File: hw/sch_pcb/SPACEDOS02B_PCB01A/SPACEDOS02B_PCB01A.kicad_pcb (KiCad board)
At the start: 2 copper layers, 38 x 200 mm, 123 parts, among them J1 MCC-SD, J10 HEADER_1x01, J11 HEADER_1x01, J12 HEADER_1x01, J13 HEADER_1x01, J14 HEADER_1x01, J15 HEADER_1x01, J16 HEADER_1x01, J17 HEADER_1x01, J18 HEADER_1x01, J19 HEADER_2x01_PARALLEL, J2 HEADER_2x01_PARALLEL, J20 HEADER_1x01, J21 HEADER_1x01, J22 HEADER_2x03, J23 HEADER_1x01, J24 HEADER_1x01, J25 HEADER_1x01, J26 HEADER_1x01, J27 HEADER_1x01, J28 SD_Card-FPS009-4200-0, J3 HEADER_2x01_PARALLEL, J4 HEADER_1x01, J5 HEADER_1x01, J6 HEADER_1x01, J7 HEADER_1x01, J8 HEADER_1x01, J9 HEADER_1x01, M6 BMI-S-210-F, M8 BMI-S-210-F, U1 OPA2314, U10 ATMEGA1284P-AU, U11 PCF85263A, U2 OPA2314, U3 ISL21080DIH312Z-TK 1V25, U4 TS7211, U5 TS5A4594, U6 AT24CS64-SSHM, U8 TPS613222ADBV, Y1 1,8432MHz, Y2 ABS07-120-32.768KHZ-T

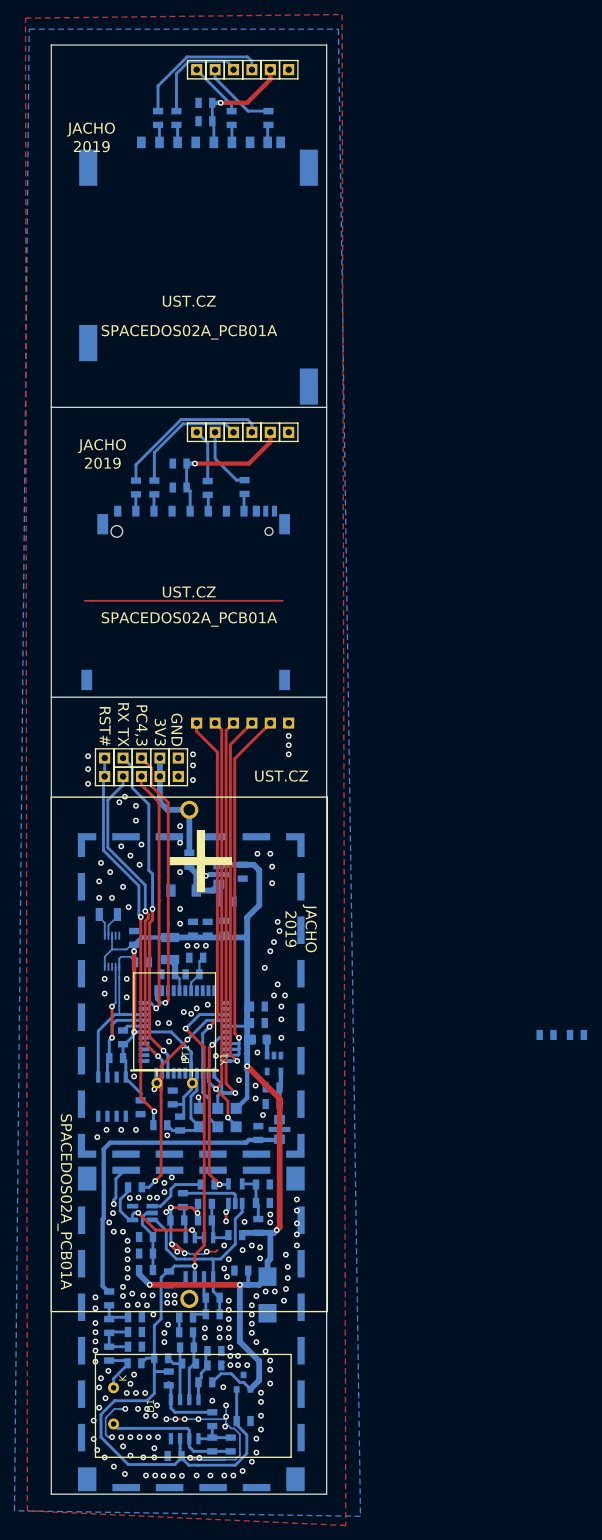
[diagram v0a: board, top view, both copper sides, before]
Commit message: Edit PCB
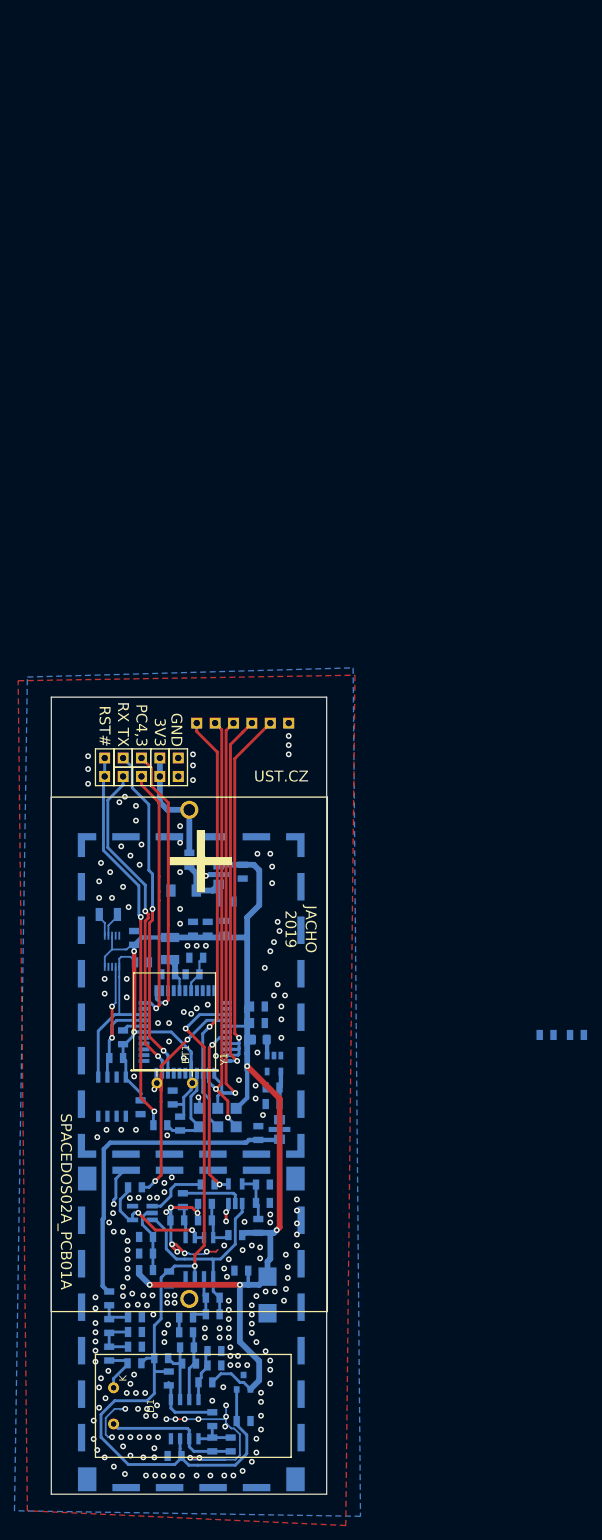
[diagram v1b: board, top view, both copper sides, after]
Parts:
- removed C22, C33: 10uF, Mlab_R:SMD-0805
- removed C25, C37: 100nF, Mlab_R:SMD-0805
- removed J1: MCC-SD, Mlab_CON:MCC-SD
- removed J14, J15, J16, J17, J18, J20, J21, J23, J24, J25, J26, J27: HEADER_1x01, Mlab_Pin_Headers:Straight_1x01
- removed J28: SD_Card-FPS009-4200-0, Mlab_CON:FPS009-4200-0
- removed R14, R16, R17, R18, R24, R25, R26, R27: 100, Mlab_R:SMD-0805
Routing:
- net GND: track 99.8 -> 72.5 mm
- net Net-(J14-Pad1): track 22.2 -> 0.00 mm
- net /cpu/SD_VDD2: track 20.9 -> 0.00 mm, vias 1 -> 0
- net Net-(J21-Pad1): track 19.5 -> 0.00 mm
- net Net-(J15-Pad1): track 16.9 -> 0.00 mm
- net /cpu/SD_VDD3: track 16.2 -> 0.00 mm, vias 1 -> 0
- net Net-(J23-Pad1): track 14.4 -> 0.00 mm
- net Net-(J26-Pad1): track 10.4 -> 0.00 mm
- net Net-(J18-Pad1): track 8.93 -> 0.00 mm
- net Net-(J25-Pad1): track 7.71 -> 0.00 mm
- net Net-(J17-Pad1): track 7.36 -> 0.00 mm
- net Net-(J28-Pad1): track 2.49 -> 0.00 mm
- net Net-(J28-Pad2): track 2.47 -> 0.00 mm
- net Net-(J28-Pad7): track 2.45 -> 0.00 mm
- net Net-(J28-Pad5): track 2.42 -> 0.00 mm
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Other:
- board size 38 x 200 mm -> 38 x 110 mm
